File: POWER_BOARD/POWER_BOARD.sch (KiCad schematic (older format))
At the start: 37 parts, among them IC1 ILQ30, J2 ARM, J3 Pyro1, J4 Pyro2, J5 Servo2, J6 Servo1, J7 Batt, J9 EXTIN, Q1 IRL40B212, Q2 IRL40B212, U1 SF-1206HH10M-2, U2 SF-1206HH10M-2, U3 AS358AP

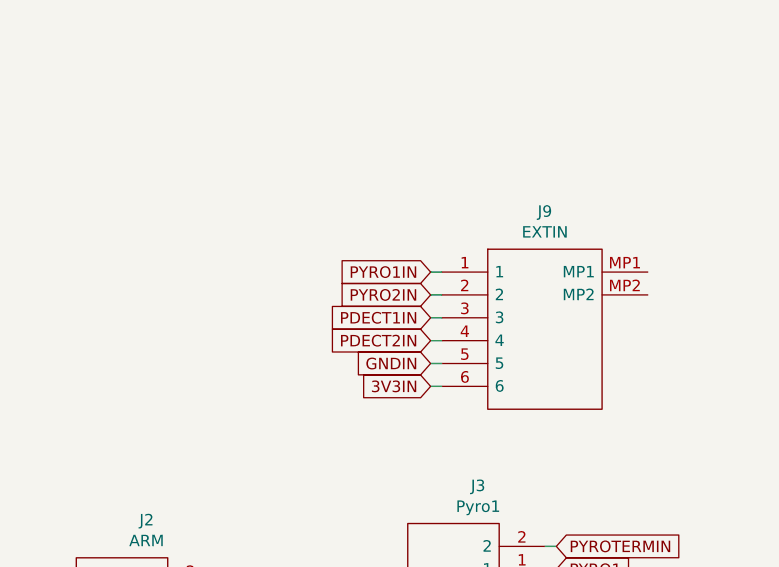
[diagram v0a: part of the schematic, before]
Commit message: duh
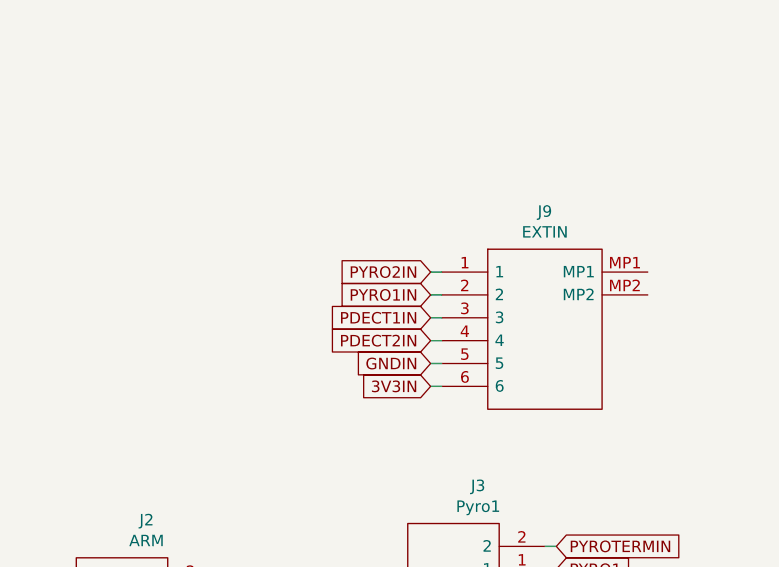
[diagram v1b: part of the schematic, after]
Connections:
- net PYRO1IN: now also J9.2; no longer J9.1
- net PYRO2IN: now also J9.1; no longer J9.2
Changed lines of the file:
@@
 Text Notes 9050 2250 0    50   ~ 0
 Ampli OP for pyro detection
+Text GLabel 2750 5350 0    50   Input ~ 0
+PYRO1IN
 Text GLabel 2750 5250 0    50   Input ~ 0
-PYRO1IN
-Text GLabel 2750 5350 0    50   Input ~ 0
 PYRO2IN
 Text GLabel 2750 5450 0    50   Input ~ 0
